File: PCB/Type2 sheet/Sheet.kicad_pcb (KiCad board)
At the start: 2 copper layers, 111.2 x 96.9 mm, 77 parts, among them P1 C_0201_0603Metric_Pad0.64x0.4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, P2 C_0201_0603Metric_Pad0.64x0.4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, P3 C_0201_0603Metric_Pad0.64x0.4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, P4 C_0201_0603Metric_Pad0.64x0.4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, P5 C_0201_0603Metric_Pad0.64x0.4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, U1 MCP9700Ax-ELT, U10 ADS7830, U11 ADS7830, U2 MCP2562-E-MF, U3 ATtiny1616-M, U5 CD74HC4067SM, U6 MCP2515-xST, U7 DRV5055A1xDBZxQ1, U8 DRV5055A1xDBZxQ1, U9 ADS7830

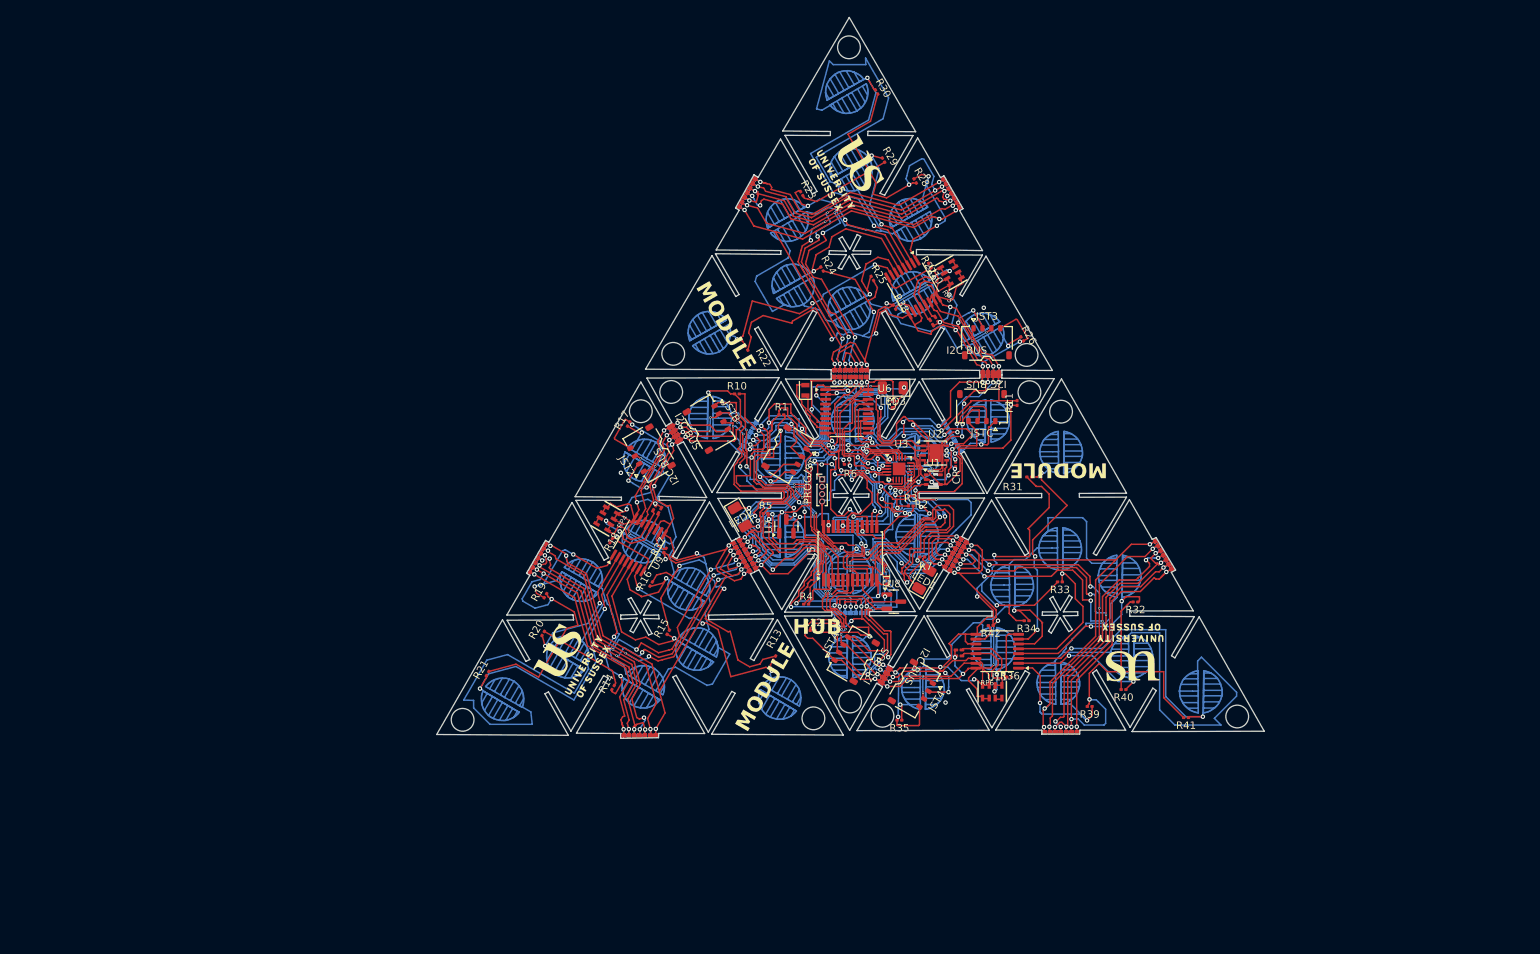
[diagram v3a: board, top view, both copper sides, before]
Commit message: sheet with mic
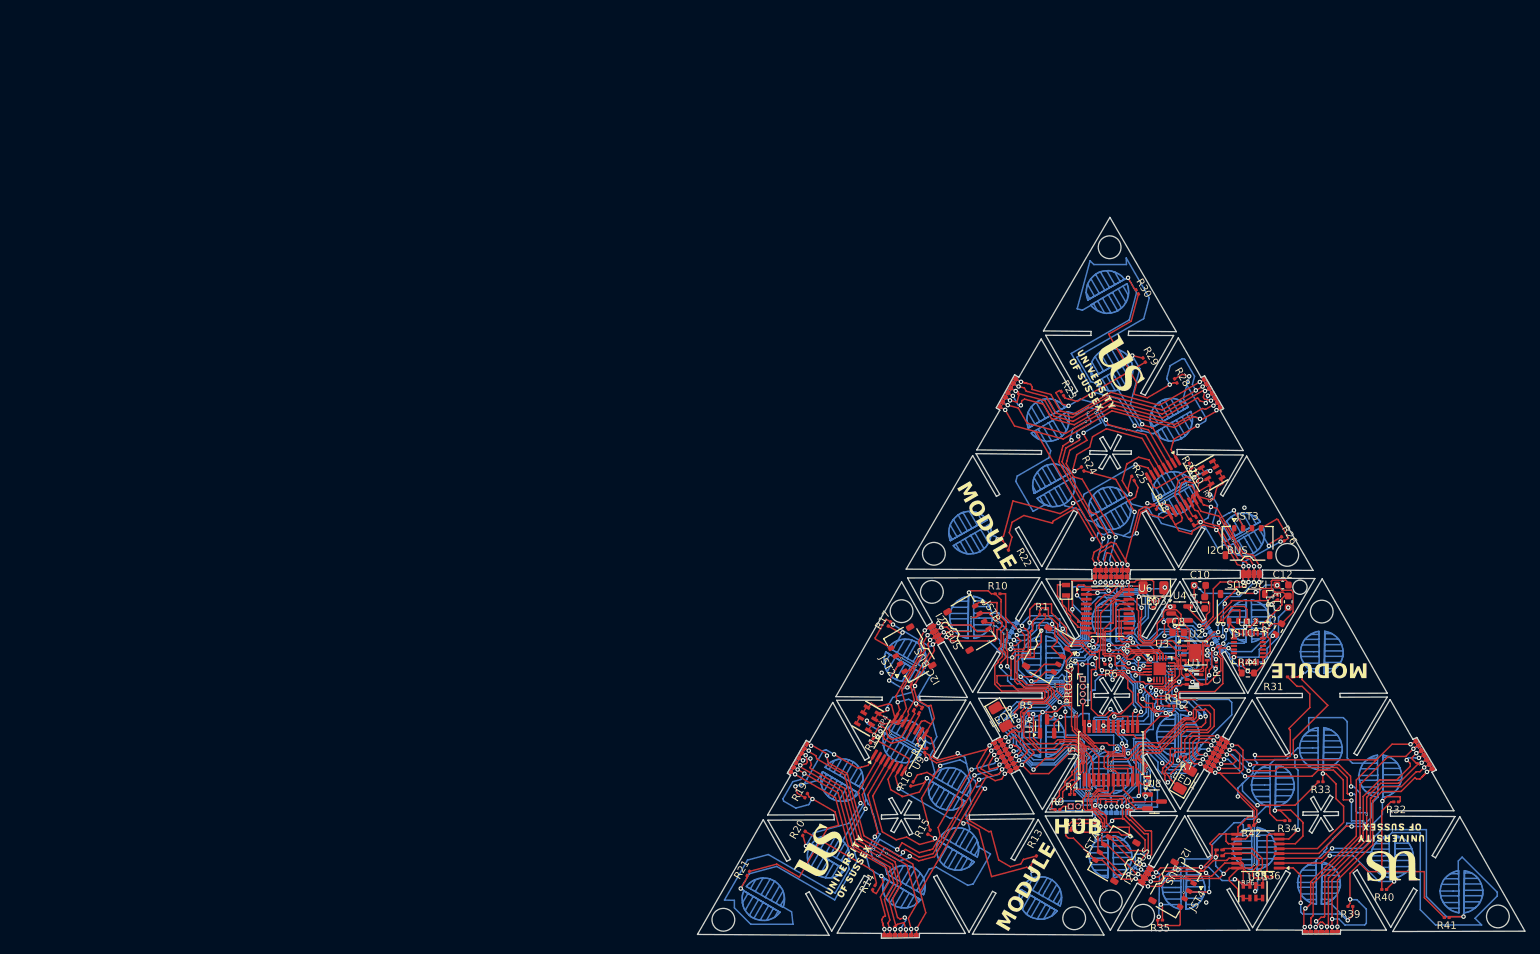
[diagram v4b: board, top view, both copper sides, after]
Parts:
- removed the P1 at (144.7, 93.0)
- removed the P1 at (145.4, 93.4)
- added C10: 0.1uF, Capacitor_SMD:C_0603_1608Metric, F.Cu at (218.0, 103.4)
- added C12: 0.1uF, Capacitor_SMD:C_0603_1608Metric, F.Cu at (229.1, 103.4)
- added C13: 0.1uF, Capacitor_SMD:C_0603_1608Metric, F.Cu at (229.9, 105.6)
- added C14: 220pF, Capacitor_SMD:C_0603_1608Metric, F.Cu at (218.6, 105.8)
- added C8: 4.7uF, Capacitor_SMD:C_0603_1608Metric, F.Cu at (215.1, 109.8)
- added P1: C_0201_0603Metric_Pad0.64x0.40mm_HandSolder, Capacitor_SMD:C_0201_0603Metric_Pad0.64x0.40mm_HandSolder, F.Cu at (179.7, 119.9)
- added P1: C_0201_0603Metric_Pad0.64x0.40mm_HandSolder, Capacitor_SMD:C_0201_0603Metric_Pad0.64x0.40mm_HandSolder, F.Cu at (180.4, 120.3)
- added R43: 4.7k, Resistor_SMD:R_0603_1608Metric, F.Cu at (228.6, 109.3)
- added R44: 4.7k, Resistor_SMD:R_0603_1608Metric, F.Cu at (224.4, 115.2)
- added R9: R9, Resistor_SMD:R_0201_0603Metric, F.Cu at (198.8, 133.6)
- added REF**: PinHeader_1x02_P1.00mm_Vertical, Connector_PinHeader_1.00mm:PinHeader_1x02_P1.00mm_Vertical, F.Cu at (200.6, 133.2)
- added U12: MPU-6050, Sensor_Motion:InvenSense_QFN-24_4x4mm_P0.5mm, F.Cu at (224.5, 111.8)
- added U4: AP2112K-3.3, Package_TO_SOT_SMD:SOT-23-5, F.Cu at (215.3, 107.2)
- R40: value R -> 1k
- R41, R42: value R -> 4.7k
- moved R20 44.2 mm to (164.8, 136.8)
- moved G*** 44.2 mm to (168.5, 140.2)
- moved JST2 44.2 mm to (179.0, 112.5)
- moved R18 44.2 mm to (173.9, 124.3)
- moved R21 44.2 mm to (157.3, 142.2)
- moved R37 44.2 mm to (181.1, 125.6)
- moved RP4 44.2 mm to (173.3, 121.3)
- moved U9 44.2 mm to (177.6, 124.8)
- moved R13 44.2 mm to (195.8, 140.1)
- moved R14 44.2 mm to (174.2, 144.1)
- moved R16 44.2 mm to (179.3, 130.1)
- moved R19 44.2 mm to (165.1, 131.7)
- moved R15 44.2 mm to (181.6, 136.6)
- moved R17 44.2 mm to (176.3, 108.6)
- moved P4 44.2 mm to (220.6, 139.0)
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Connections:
- R22 pad 2: Net-(U9-CH0) -> Net-(U10-CH1)
- R23 pad 2: Net-(U9-CH1) -> Net-(U10-CH2)
- R24 pad 2: Net-(U9-CH2) -> Net-(U10-CH3)
- R25 pad 2: Net-(U9-CH3) -> Net-(U10-CH4)
- R26 pad 2: Net-(U9-CH4) -> Net-(U10-CH5)
- R27 pad 2: Net-(U9-CH5) -> Net-(U10-CH6)
- R28 pad 2: Net-(U9-CH6) -> Net-(U10-CH7)
- R29 pad 1: unconnected-(R20-Pad1) -> Net-(MK1--)
- R29 pad 2: Net-(U9-CH7) -> Net-(U11-CH0)
- R30 pad 2: Net-(U10-CH0) -> Net-(U11-CH1)
- R31 pad 2: Net-(U9-CH0) -> Net-(U11-CH2)
- R32 pad 2: Net-(U9-CH1) -> Net-(U11-CH3)
- R33 pad 2: Net-(U9-CH2) -> Net-(U11-CH4)
- R34 pad 2: Net-(U9-CH3) -> Net-(U11-CH5)
- R35 pad 2: Net-(U9-CH4) -> Net-(U11-CH6)
- R36 pad 2: Net-(U9-CH5) -> Net-(U11-CH7)
- R38 pad 2: Net-(U9-REFin/REFout) -> Net-(U10-REFin/REFout)
- R39 pad 1: Net-(MK1--) -> Net-(U1-V_{DD})
- R39 pad 2: Net-(U9-CH6) -> Net-(U11-REFin/REFout)
- R40 pad 1: unconnected-(R20-Pad1) -> +3V3
- R40 pad 2: Net-(U9-CH7) -> Net-(D4-A)
- R41 pad 1: Net-(MK1--) -> +3V3
- R41 pad 2: Net-(U10-CH0) -> /SCL
- R42 pad 1: Net-(U1-V_{DD}) -> +3V3
- R42 pad 2: Net-(U9-REFin/REFout) -> /SDA
- U5 pad 18: Net-(U4-ZOUT) -> unconnected-(U5-I13-Pad18)
- U5 pad 21: Net-(U4-YOUT) -> unconnected-(U5-I10-Pad21)
- U5 pad 22: Net-(U4-XOUT) -> unconnected-(U5-I9-Pad22)
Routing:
- net (no net): track 3022.7 -> 2905.6 mm, vias 182 -> 183
- net Net-(U11-CH2): track 0.00 -> 52.8 mm, vias 0 -> 2
- net +3V3: track 0.00 -> 41.6 mm, vias 0 -> 4
- net Net-(U11-CH1): track 0.00 -> 33.2 mm, vias 0 -> 2
- net Net-(MK1--): track 495.7 -> 464.2 mm, vias 47 -> 45
- net Net-(U11-CH7): track 0.00 -> 22.7 mm, vias 0 -> 1
- net Net-(U1-V_{DD}): track 472.8 -> 493.2 mm, vias 56 -> 58
- net unconnected-(R20-Pad1): track 39.0 -> 19.5 mm, vias 4 -> 2
- net GND: track 0.00 -> 15.0 mm
- net Net-(U5-I5): track 88.6 -> 102.4 mm
- net Net-(U5-I14): track 11.7 -> 25.5 mm
- net Net-(U5-I12): track 16.9 -> 30.7 mm
- net Net-(U5-I1): track 84.5 -> 97.3 mm, vias 7 -> 8
- net Net-(U5-I6): track 19.5 -> 31.6 mm
- net Net-(U12-REGOUT): track 0.00 -> 10.4 mm, vias 0 -> 2
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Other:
- outline, holes or cut-outs redrawn

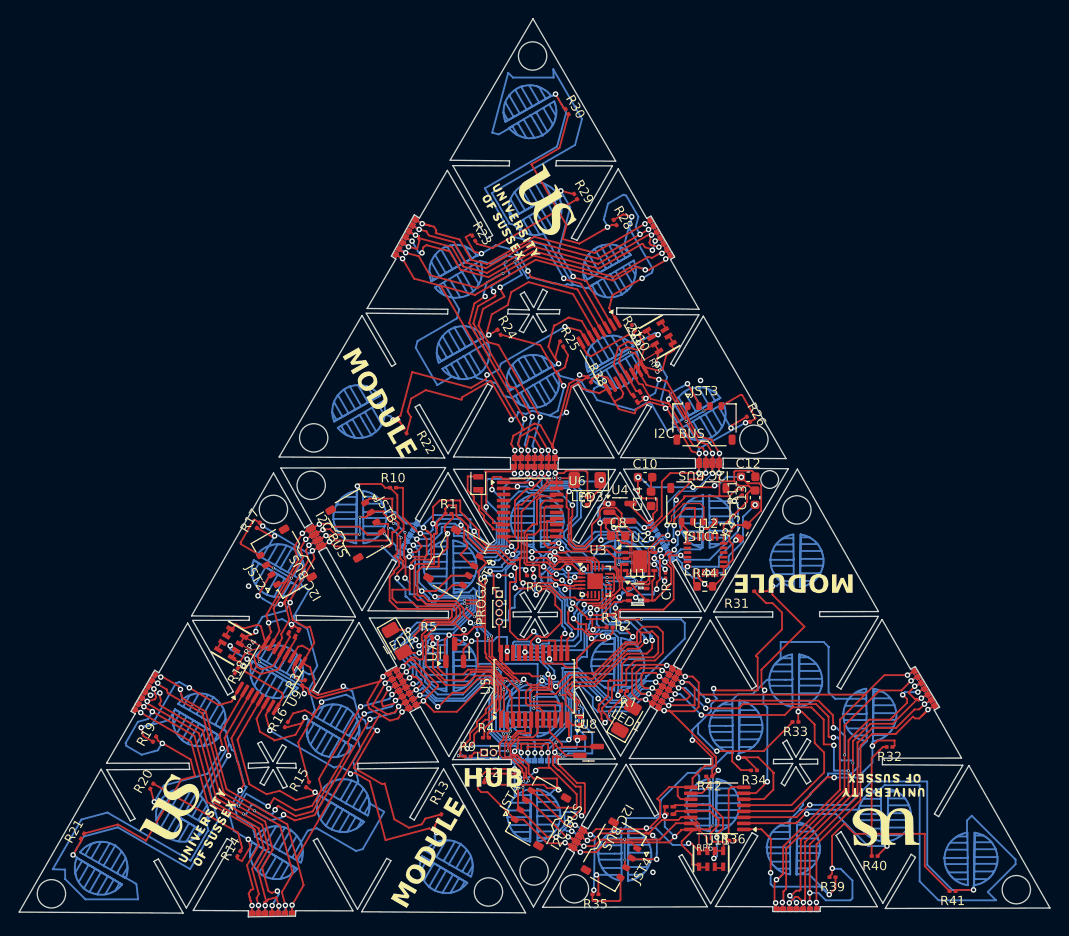
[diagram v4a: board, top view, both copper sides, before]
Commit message: sheet usable
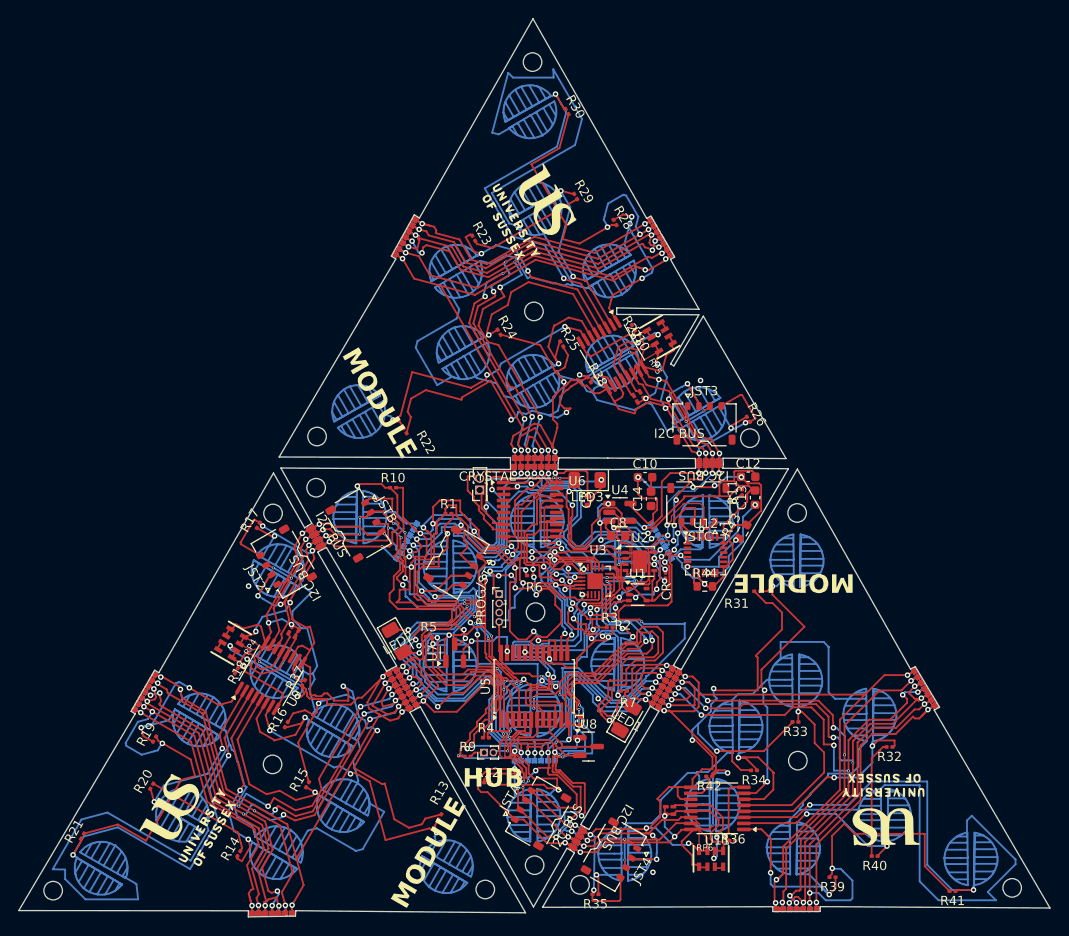
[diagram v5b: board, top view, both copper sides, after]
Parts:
- removed crystal: Crystal_SMD_2012-2Pin_2.0x1.2mm, Crystal:Crystal_SMD_2012-2Pin_2.0x1.2mm
- added CRYSTAL: Crystal 8MHz, Connector_PinHeader_1.27mm:PinHeader_2x01_P1.27mm_Vertical, F.Cu at (200.2, 104.8)
- R40: value 1k -> R
- R41: value 4.7k -> R
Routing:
- net Net-(MK1--): track 464.2 -> 530.0 mm, vias 45 -> 49
- net Net-(U5-I1): track 97.3 -> 35.9 mm, vias 8 -> 4
- net Net-(U1-V_{DD}): track 493.2 -> 499.0 mm
- net (no net): track 2905.6 -> 2907.1 mm
- net Net-(U9-CH0): track 136.0 -> 136.8 mm
- net Net-(U10-SCL): track 196.9 -> 197.5 mm
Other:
- board size 111.2 x 96.9 mm -> 111.3 x 96.9 mm
